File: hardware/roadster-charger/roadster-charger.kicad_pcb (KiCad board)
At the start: 4 copper layers, 74.4 x 50.2 mm, 107 parts, among them J1 USB4505-03-0-A, J2 USB4505-03-0-A, J3 54-00166, Q1 CSD19532Q5B, U1 MPM3606AGQV-P, U10 DAC70501ZDQFT, U11 PI3740-00-LGIZ, U2 ESP32-C3-MINI-1, U3 INA168, U4 OPA340NA, U5 FUSB307BMPX, U6 LM75B, U7 LM5050-1, U8 INA168, U9 OPA340NA

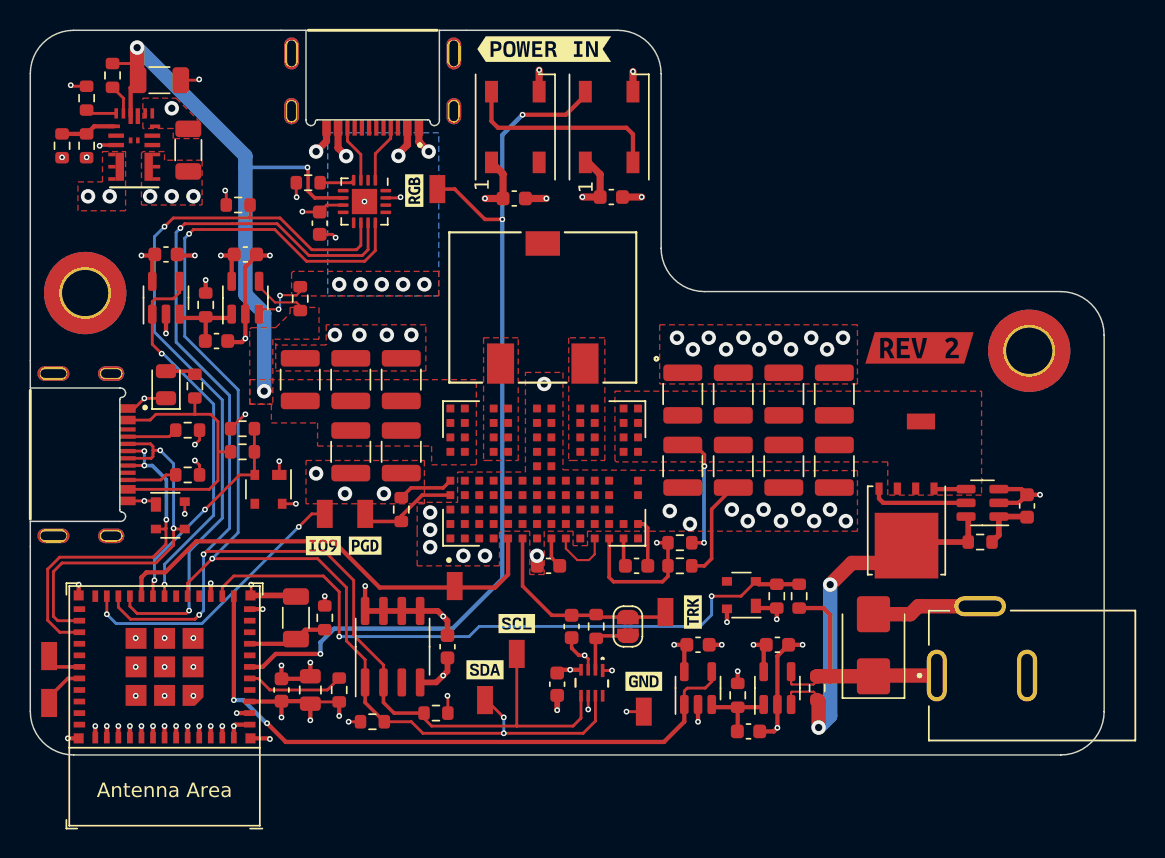
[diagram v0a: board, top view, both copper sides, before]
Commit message: use track cleanup tool
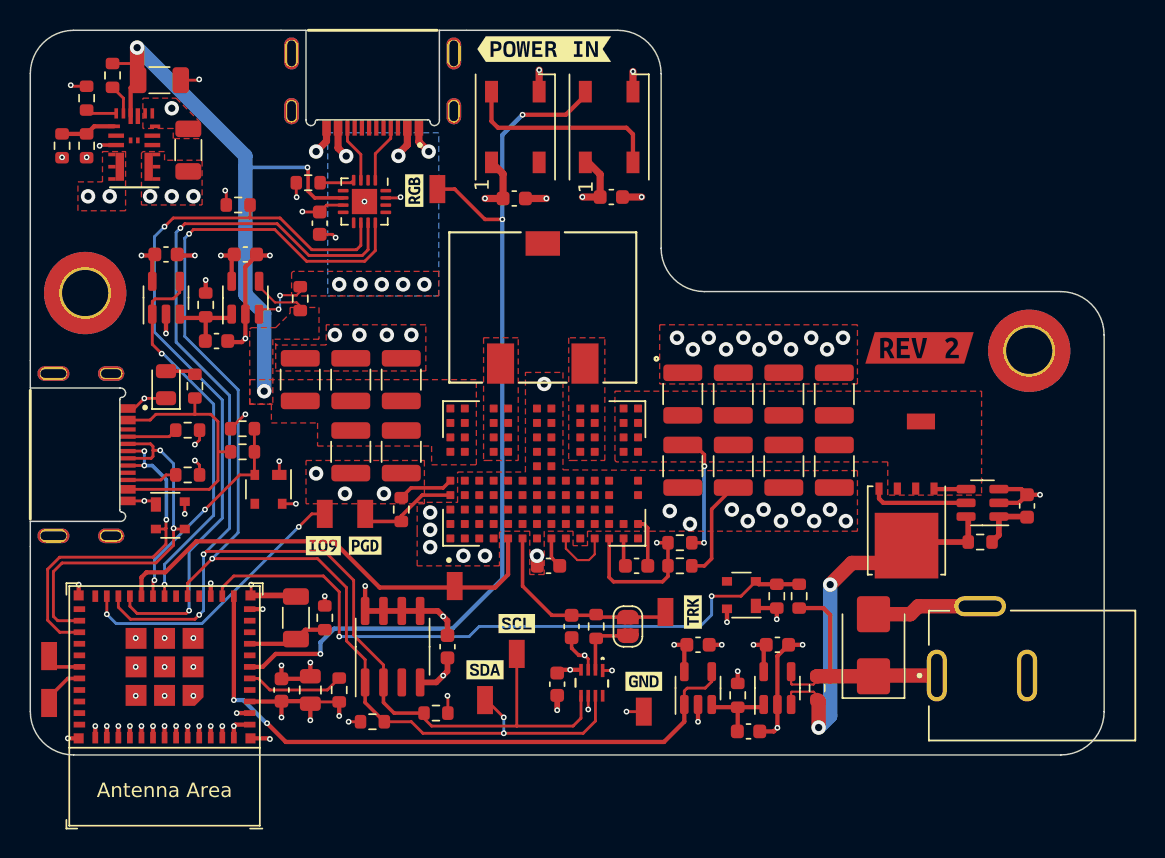
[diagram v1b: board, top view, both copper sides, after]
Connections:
- J1 pad S1: GND -> unconnected-(J1-SHELL_GND-PadS1)_1
- J1 pad S2: GND -> unconnected-(J1-SHELL_GND-PadS1)_3
- J1 pad S3: GND -> unconnected-(J1-SHELL_GND-PadS1)
- J1 pad S4: GND -> unconnected-(J1-SHELL_GND-PadS1)_2
- J2 pad S1: GND -> unconnected-(J2-SHELL_GND-PadS1)_1
- J2 pad S2: GND -> unconnected-(J2-SHELL_GND-PadS1)_2
- J2 pad S3: GND -> unconnected-(J2-SHELL_GND-PadS1)_3
- J2 pad S4: GND -> unconnected-(J2-SHELL_GND-PadS1)
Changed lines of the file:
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@@
 	(net 91 "Net-(U11-VDIFF)")
 	(net 92 "unconnected-(U11-SYNCO-PadC1)")
+	(net 93 "unconnected-(J1-SHELL_GND-PadS1)")
+	(net 94 "unconnected-(J1-SHELL_GND-PadS1)_1")
+	(net 95 "unconnected-(J1-SHELL_GND-PadS1)_2")
+	(net 96 "unconnected-(J1-SHELL_GND-PadS1)_3")
+	(net 97 "unconnected-(J2-SHELL_GND-PadS1)")
+	(net 98 "unconnected-(J2-SHELL_GND-PadS1)_1")
+	(net 99 "unconnected-(J2-SHELL_GND-PadS1)_2")
+	(net 100 "unconnected-(J2-SHELL_GND-PadS1)_3")
 	(footprint "kibuzzard-657BB005"
 		(layer "F.Cu")
@@
 			(layers "*.Cu")
 			(remove_unused_layers no)
-			(net 2 "GND")
+			(net 98 "unconnected-(J2-SHELL_GND-PadS1)_1")
 			(pinfunction "SHELL_GND")
-			(pintype "power_in")
+			(pintype "power_in+no_connect")
 		)
 		(pad "S2" thru_hole oval
@@
 			(layers "*.Cu")
 			(remove_unused_layers no)
-			(net 2 "GND")
+			(net 99 "unconnected-(J2-SHELL_GND-PadS1)_2")
 			(pinfunction "SHELL_GND")
-			(pintype "power_in")
+			(pintype "power_in+no_connect")
 		)
 		(pad "S3" thru_hole oval
@@
 			(layers "*.Cu")
 			(remove_unused_layers no)
-			(net 2 "GND")
+			(net 100 "unconnected-(J2-SHELL_GND-PadS1)_3")
 			(pinfunction "SHELL_GND")
-			(pintype "power_in")
+			(pintype "power_in+no_connect")
 		)
 		(pad "S4" thru_hole oval
@@
 			(layers "*.Cu")
 			(remove_unused_layers no)
-			(net 2 "GND")
+			(net 97 "unconnected-(J2-SHELL_GND-PadS1)")
 			(pinfunction "SHELL_GND")
-			(pintype "power_in")
+			(pintype "power_in+no_connect")
 		)
 		(model "${KIPRJMOD}/components/USB4505-03-0-A_REVA/USB4505-03-0-A_REVA.step"
@@
 			(layers "*.Cu")
 			(remove_unused_layers no)
-			(net 2 "GND")
+			(net 94 "unconnected-(J1-SHELL_GND-PadS1)_1")
 			(pinfunction "SHELL_GND")
-			(pintype "power_in")
+			(pintype "power_in+no_connect")
 		)
 		(pad "S2" thru_hole oval
@@
 			(layers "*.Cu")
 			(remove_unused_layers no)
-			(net 2 "GND")
+			(net 96 "unconnected-(J1-SHELL_GND-PadS1)_3")
 			(pinfunction "SHELL_GND")
-			(pintype "power_in")
+			(pintype "power_in+no_connect")
 		)
 		(pad "S3" thru_hole oval
@@
 			(layers "*.Cu")
 			(remove_unused_layers no)
-			(net 2 "GND")
+			(net 93 "unconnected-(J1-SHELL_GND-PadS1)")
 			(pinfunction "SHELL_GND")
-			(pintype "power_in")
+			(pintype "power_in+no_connect")
 		)
 		(pad "S4" thru_hole oval
@@
 			(layers "*.Cu")
 			(remove_unused_layers no)
-			(net 2 "GND")
+			(net 95 "unconnected-(J1-SHELL_GND-PadS1)_2")
 			(pinfunction "SHELL_GND")
-			(pintype "power_in")
+			(pintype "power_in+no_connect")
 		)
 		(model "${KIPRJMOD}/components/USB4505-03-0-A_REVA/USB4505-03-0-A_REVA.step"
@@
 				(font
 					(size 0.001 0.001)
+					(thickness 0.15)
 				)
 			)
@@
 				(font
 					(size 0.001 0.001)
+					(thickness 0.15)
 				)
 			)
@@
 	)
 	(segment
-		(start 186.75 158.35)
-		(end 186.8 158.3)
-		(width 0.2)
-		(layer "F.Cu")
-		(net 2)
-	)
-	(segment
 		(start 190 158.3)
 		(end 190 157.5)
@@
 	)
 	(segment
-		(start 204.5 157.2)
-		(end 204.45 157.2)
-		(width 0.2)
-		(layer "F.Cu")
-		(net 3)
-	)
-	(segment
 		(start 190 124.9)
 		(end 190.575 124.9)
@@
 	)
 	(segment
-		(start 194.45 130.875)
-		(end 194.425 130.9)
-		(width 0.3)
-		(layer "F.Cu")
-		(net 5)
-	)
-	(segment
 		(start 194.45 129.225)
 		(end 196.0625 129.225)
@@
 	)
 	(segment
-		(start 190.2 139)
-		(end 190.2 139.4495)
-		(width 0.2)
-		(layer "B.Cu")
-		(net 18)
-	)
-	(segment
 		(start 190.7495 139.4495)
 		(end 190.2 139.4495)
@@
 	(segment
 		(start 190.2 138.4495)
-		(end 190.2 139)
+		(end 190.2 139.4495)
 		(width 0.2)
 		(layer "B.Cu")
@@
 	)
 	(segment
-		(start 190.8 138.6)
+		(start 190.8 138.4)
 		(end 190.8 138.82)
 		(width 0.2)
@@
 	)
 	(segment
-		(start 190.8 138.4)
-		(end 190.8 138.6)
-		(width 0.2)
-		(layer "F.Cu")
-		(net 19)
-	)
-	(segment
 		(start 190.63 137.95)
 		(end 190.8 138.12)
@@
 	)
 	(segment
-		(start 198.1245 128.6245)
-		(end 198.1 128.6)
-		(width 0.15)
-		(layer "F.Cu")
-		(net 24)
-	)
-	(segment
 		(start 200.75 127.65)
 		(end 199.6255 127.65)
@@
 	)
 	(segment
-		(start 199.399999 122.7)
-		(end 197.4 122.7)
+		(start 193 122.7)
+		(end 199.399999 122.7)
 		(width 0.2)
 		(layer "F.Cu")
@@
 	)
 	(segment
-		(start 196.6 122.7)
-		(end 196.3 122.7)
-		(width 0.2)
-		(layer "F.Cu")
-		(net 45)
-	)
-	(segment
 		(start 204.7 147.4)
 		(end 204.7 151.2)
@@
 	)
 	(segment
-		(start 197.4 122.7)
-		(end 196.6 122.7)
-		(width 0.2)
-		(layer "F.Cu")
-		(net 45)
-	)
-	(segment
 		(start 207.5 156.6)
 		(end 209.575 156.6)
@@
 	)
 	(segment
-		(start 196.3 122.7)
-		(end 193 122.7)
-		(width 0.2)
-		(layer "F.Cu")
-		(net 45)
-	)
-	(segment
 		(start 205.3 124.9)
 		(end 201.6 124.9)
@@
 		(width 0.25)
 		(layer "F.Cu")
-		(net 90)
-	)
-	(segment
-		(start 219.85 149.775)
-		(end 219.8 149.825)
-		(width 0.25)
-		(layer "F.Cu")
